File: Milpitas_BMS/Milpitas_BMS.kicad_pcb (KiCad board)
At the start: 4 copper layers, 94 x 103.4 mm, 318 parts, among them J100 JTAG, J102 DIAGS_CON, J104 CAN_CONN, J400 CHG INPUT, J401 POWER_OUTPUT, J402 BATT_PWR_INPUT, J500 SOUTH CELL CONN, J501 NORTH CELL CONN, Q400 RU1J002YNTCL, Q401 RU1J002YNTCL, Q402 RU1J002YNTCL, SW100 SW_SPST, SW101 SW_SPST, U1 BQ79606, U100 MIC5283-3.3ML-TR, U101 STM32F303RETx, U102 SN65HVD232, U200 BQ79606, U400 ACS711, U401 BTS6163DAUMA1, U402 ACS711, U403 BTS6163DAUMA1, U404 BTS6163DAUMA1, U405 ACS711, Y1 32.768kHz, Y2 32MHz

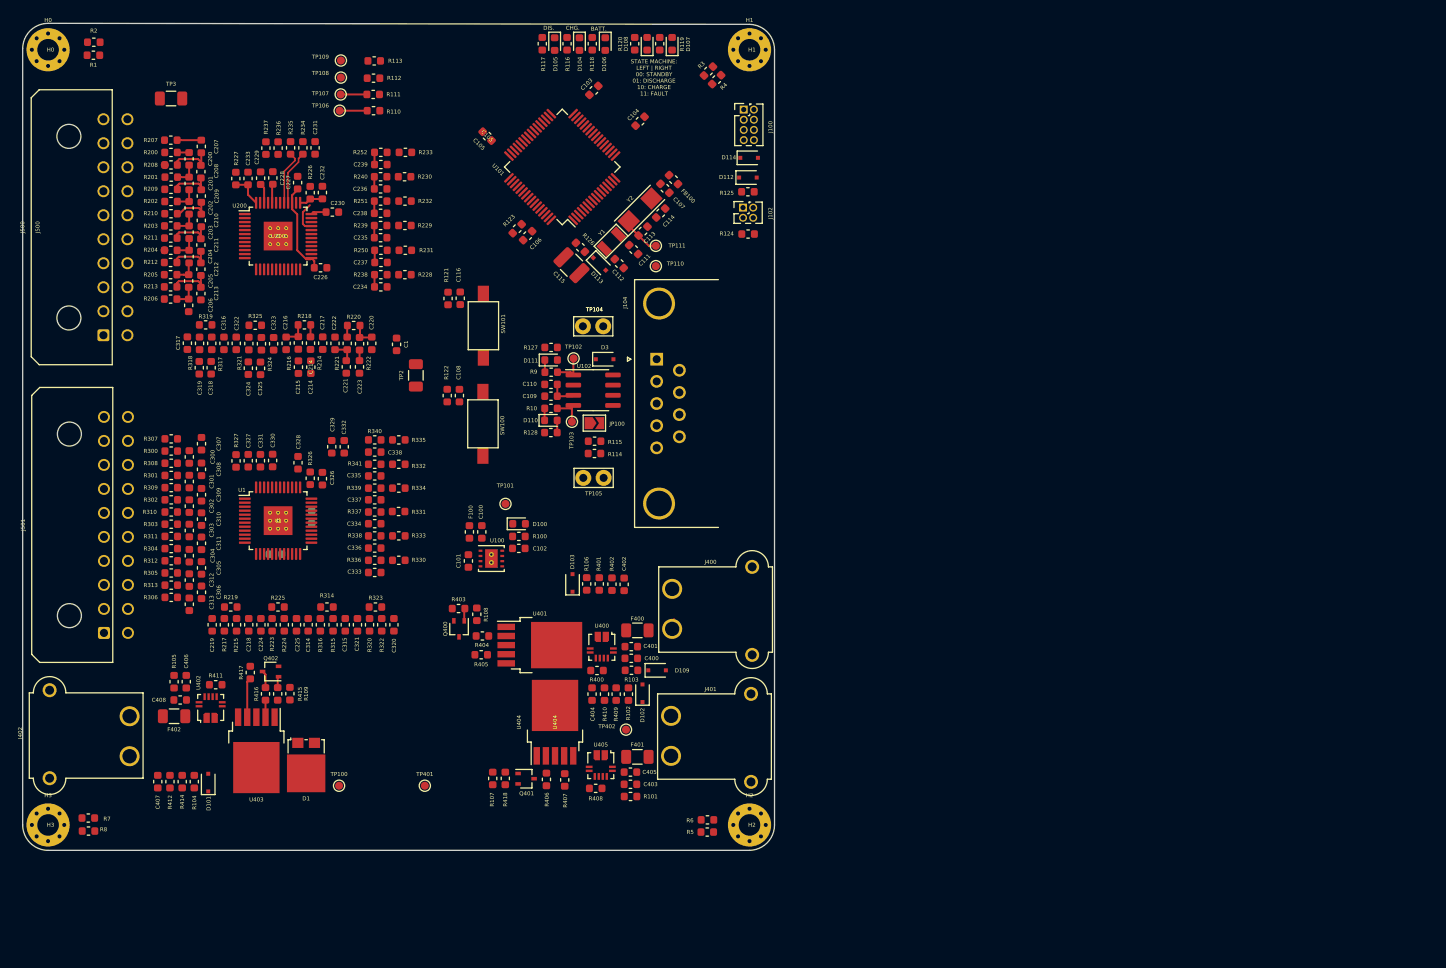
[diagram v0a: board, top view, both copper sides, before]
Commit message: First pass routing
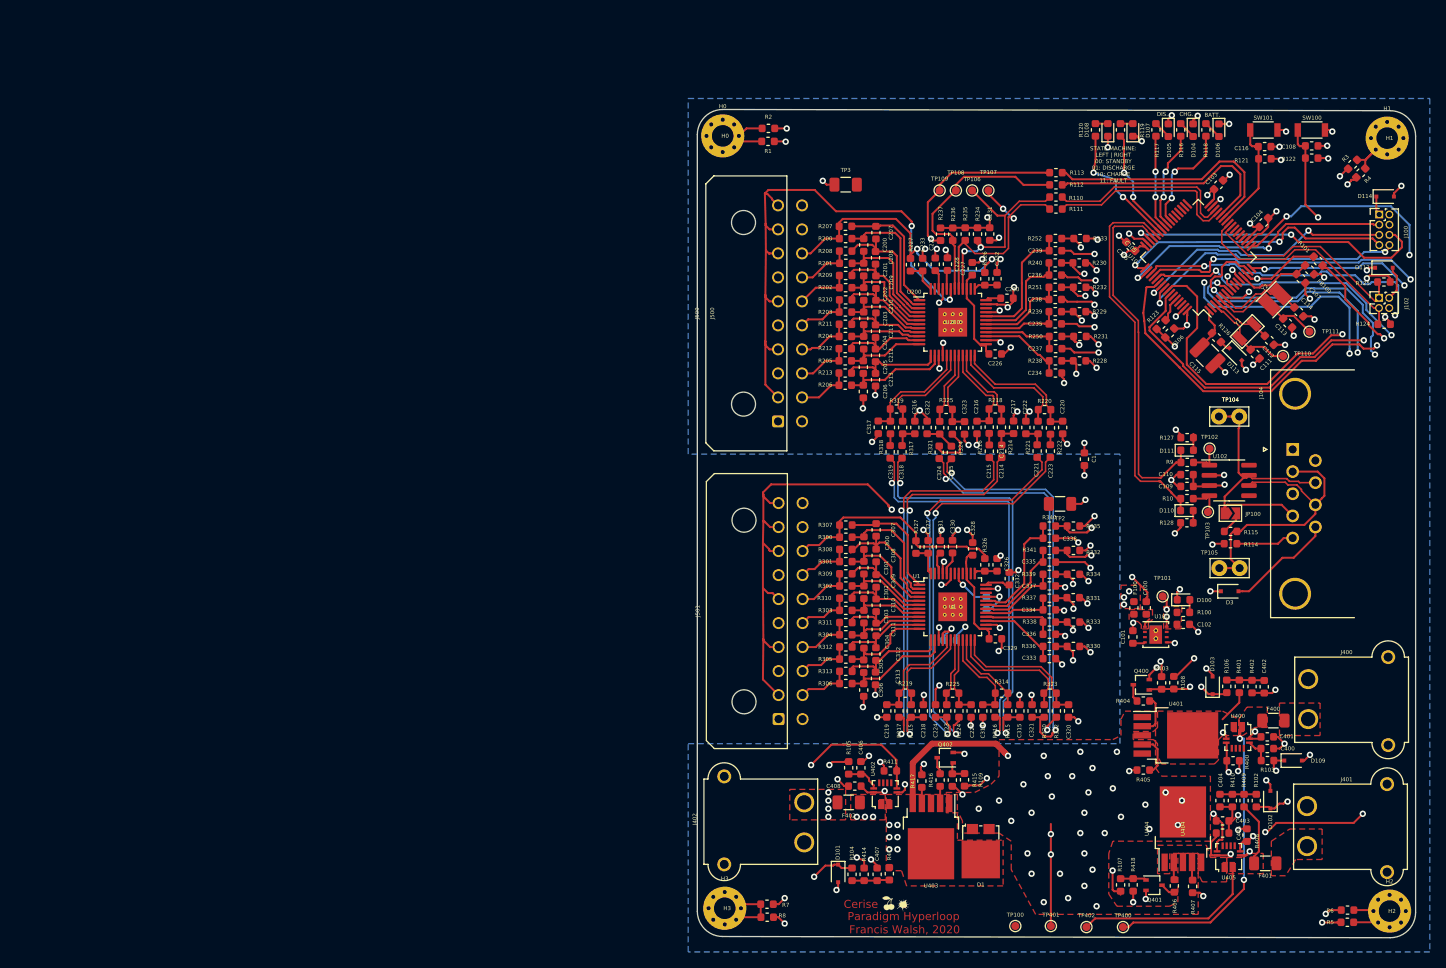
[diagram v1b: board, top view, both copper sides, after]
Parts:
- added G***: LOGO, Pics:rear_anime_ss, B.Cu at (135.4, 70.7)
- added G***: LOGO, Pics:spirograph_soldermask, F.Cu at (117.0, 146.1)
- added G***: LOGO, Pics:gunshot_logo, F.Cu at (127.3, 144.7)
- added G***: LOGO, Pics:cherry_logo, F.Cu at (125.3, 144.4)
- added TP400: CHARGER, TestPoint:TestPoint_Pad_D1.0mm, F.Cu at (154.7, 147.4)
- SW100, SW101: footprint Milpitas_BMS:KSR223GLFG -> Milpitas_BMS:B3U-1100P
- Y2: value 32MHz -> 16MHz; footprint Milpitas_BMS:NX5032GA -> Milpitas_BMS:NX3225GB
- moved R122 112.1 mm to (178.3, 51.3), turned to 180 degrees
- moved C108 111.0 mm to (178.3, 49.7), turned to 0 degrees
- moved R101 108.9 mm to (179.1, 64.1), turned to 315 degrees
- moved SW100 106.7 mm to (176.5, 47.8), turned to 0 degrees
- moved R121 103.6 mm to (172.4, 51.4), turned to 180 degrees
- moved SW101 103.5 mm to (174.0, 47.8), turned to 180 degrees
- moved C116 102.3 mm to (172.4, 49.8), turned to 0 degrees
- moved C407 90.7 mm to (124.0, 140.8), turned to 90 degrees
- moved R412 90.7 mm to (125.5, 140.7), turned to 90 degrees
- moved R403 88.4 mm to (159.5, 116.9), turned to 90 degrees
- moved R108 87.5 mm to (161.0, 116.8)
- moved C1 87.2 mm to (149.9, 88.9)
- moved C215 87.0 mm to (138.0, 87.9)
- moved C216 87.0 mm to (136.4, 84.9)
- moved C217 87.0 mm to (141.0, 84.9)
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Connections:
- C111 pad 1: /MCU/XTAL32_IN_P -> /MCU/XTAL32_P
- C112 pad 1: /MCU/XTAL32_IN_N -> /MCU/XTAL32_N
- D110 pad 1: /MCU/CAN_RX_N -> /MCU/CAN_UART_N
- D111 pad 1: /MCU/CAN_TX_P -> /MCU/CAN_UART_P
- J100 pad 2: /MCU/JTAG_TDI -> GND
- J100 pad 3: GND -> /MCU/JTAG_TDI
- J102 pad 1: /MCU/DIAGS_P -> /MCU/DIAGS_N
- J102 pad 3: /MCU/DIAGS_N -> /MCU/DIAGS_P
- J104 pad 1: Net-(D3-Pad2) -> Net-(J104-Pad1)
- J104 pad 2: /MCU/CAN_P -> /MCU/CAN_N
- J104 pad 3: /MCU/CAN_N -> Net-(J104-Pad3)
- J104 pad 6: Net-(J104-Pad6) -> GND
- J104 pad 7: Net-(J104-Pad7) -> /MCU/CAN_P
- J104 pad 9: GND -> Net-(D3-Pad2)
- J500 pad 1: Net-(J500-Pad1) -> SOUTH_THERM1_N
- J500 pad 10: Net-(J500-Pad10) -> SOUTH_THERM1_P
- J500 pad 19: Net-(J500-Pad19) -> SOUTH_THERM5_N
- J500 pad 2: Net-(J500-Pad2) -> SOUTH_THERM1_P
- J500 pad 20: Net-(J500-Pad20) -> SOUTH_THERM6_N
- J500 pad 3: Net-(J500-Pad3) -> SOUTH_THERM2_N
- J500 pad 4: Net-(J500-Pad4) -> SOUTH_THERM1_P
- J500 pad 5: Net-(J500-Pad5) -> SOUTH_THERM3_N
- J500 pad 6: Net-(J500-Pad6) -> SOUTH_THERM1_P
- J500 pad 7: Net-(J500-Pad7) -> SOUTH_THERM4_N
- J500 pad 8: Net-(J500-Pad8) -> SOUTH_THERM1_P
- J500 pad 9: Net-(J500-Pad9) -> SOUTH_THERM1_P
- J501 pad 1: NORTH_CELL_6 -> NORTH_THERM1_N
- J501 pad 11: NORTH_THERM2_N -> Net-(J501-Pad11)
- J501 pad 12: NORTH_THERM1_P -> NORTH_CELL_0
- J501 pad 13: NORTH_THERM3_N -> NORTH_CELL_1
- J501 pad 14: NORTH_THERM1_P -> NORTH_CELL_2
- J501 pad 15: NORTH_THERM4_N -> NORTH_CELL_3
- J501 pad 16: NORTH_THERM1_P -> NORTH_CELL_4
- J501 pad 17: NORTH_THERM5_N -> NORTH_CELL_5
- J501 pad 18: NORTH_THERM1_P -> NORTH_CELL_6
- J501 pad 19: NORTH_THERM6_N -> NORTH_THERM5_N
- J501 pad 2: NORTH_CELL_5 -> NORTH_THERM1_P
- J501 pad 20: Net-(J501-Pad20) -> NORTH_THERM6_N
- J501 pad 3: NORTH_CELL_5 -> NORTH_THERM2_N
- J501 pad 4: NORTH_CELL_3 -> NORTH_THERM1_P
- J501 pad 5: NORTH_CELL_2 -> NORTH_THERM3_N
- J501 pad 6: SOUTH_CELL_1 -> NORTH_THERM1_P
- J501 pad 7: NORTH_CELL_0 -> NORTH_THERM4_N
- J501 pad 9: NORTH_THERM1_N -> NORTH_THERM1_P
- R10 pad 1: /MCU/CAN_RX_N -> /MCU/CAN_UART_N
- R124 pad 1: /MCU/DIAGS_N -> /MCU/DIAGS_P
- R125 pad 1: /MCU/DIAGS_P -> /MCU/DIAGS_N
- R302 pad 2: NORTH_CELL_5 -> NORTH_CELL_4
- R305 pad 2: SOUTH_CELL_1 -> NORTH_CELL_1
- R309 pad 2: NORTH_CELL_5 -> NORTH_CELL_4
- R312 pad 2: SOUTH_CELL_1 -> NORTH_CELL_1
- R326 pad 2: +BATT -> NORTH_CELL_6
- R327 pad 2: +BATT -> NORTH_CELL_6
- R9 pad 1: /MCU/CAN_TX_P -> /MCU/CAN_UART_P
- TP110 pad 1: /MCU/XTAL32_IN_P -> /MCU/XTAL32_P
- U101 pad 14: Net-(U101-Pad14) -> /MCU/I_DIS_J
- U101 pad 15: Net-(U101-Pad15) -> /MCU/V_DIS_J
- U101 pad 16: Net-(U101-Pad16) -> /MCU/I_BATT_J
- U101 pad 17: Net-(U101-Pad17) -> /MCU/V_BATT_J
- U101 pad 24: /MCU/STM32_UART_J_N -> /MCU/DIAGS_N
- U101 pad 25: /MCU/STM32_UART_J_P -> /MCU/DIAGS_P
- U101 pad 26: Net-(U101-Pad26) -> /MCU/USR_BUTTON
- U101 pad 27: Net-(U101-Pad27) -> /MCU/BMS_WAKEUP_J
- U101 pad 28: Net-(U101-Pad28) -> /MCU/~BMS_FAULT_J
- U101 pad 29: /MCU/DIAGS_P -> /MCU/STM32_UART_J_N
- U101 pad 3: /MCU/XTAL32_IN_P -> /MCU/XTAL32_P
- U101 pad 30: /MCU/DIAGS_N -> /MCU/STM32_UART_J_P
- U101 pad 39: Net-(U101-Pad39) -> /MCU/BATT_LED
- U101 pad 4: /MCU/XTAL32_IN_N -> /MCU/XTAL32_N
- U101 pad 40: Net-(U101-Pad40) -> /MCU/CHG_LED
- U101 pad 41: Net-(U101-Pad41) -> /MCU/DIS_LED
- U101 pad 42: Net-(U101-Pad42) -> /MCU/SM0
- U101 pad 43: Net-(U101-Pad43) -> /MCU/SM1
- U101 pad 44: /MCU/CAN_RX_P -> /MCU/CAN_UART_N
- U101 pad 45: /MCU/CAN_TX_N -> /MCU/CAN_UART_P
- U101 pad 5: /MCU/XTAL32_IN_P -> /MCU/XTAL_P
- U101 pad 51: Net-(U101-Pad51) -> /MCU/BATT_ON_J
- U101 pad 52: Net-(U101-Pad52) -> BATT_FAULT
- U101 pad 53: Net-(U101-Pad53) -> /MCU/DIS_ON_J
- U101 pad 54: Net-(U101-Pad54) -> DIS_FAULT
- U101 pad 57: Net-(U101-Pad57) -> /MCU/CHG_ON_J
- U101 pad 58: Net-(U101-Pad58) -> CHG_FAULT
- U101 pad 6: /MCU/XTAL32_IN_N -> /MCU/XTAL_N
- U101 pad 8: Net-(U101-Pad8) -> /MCU/I_CHG_J
- U101 pad 9: Net-(U101-Pad9) -> /MCU/V_CHG_J
- Y1 pad 1: /MCU/XTAL32_IN_P -> /MCU/XTAL32_P
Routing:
- net BATT_FAULT: track 0.00 -> 223.7 mm, vias 0 -> 3
- net /MCU/I_BATT_J: track 0.00 -> 194.2 mm, vias 0 -> 3
- net /MCU/V_BATT_J: track 0.00 -> 186.1 mm, vias 0 -> 3
- net GND: track 0.00 -> 184.5 mm, vias 0 -> 99
- net /MCU/BATT_ON_J: track 0.00 -> 178.4 mm, vias 0 -> 3
- net /MCU/DIS_ON_J: track 0.00 -> 144.5 mm, vias 0 -> 3
- net DIS_FAULT: track 0.00 -> 120.1 mm, vias 0 -> 4
- net CHG_FAULT: track 0.00 -> 115.3 mm, vias 0 -> 2
- net /MCU/V_DIS_J: track 0.00 -> 105.0 mm, vias 0 -> 3
- net /MCU/V_CHG_J: track 0.00 -> 101.5 mm, vias 0 -> 4
- net /MCU/CHG_ON_J: track 0.00 -> 101.1 mm, vias 0 -> 2
- net I_DIS: track 0.00 -> 100.3 mm, vias 0 -> 2
- net /MCU/I_CHG_J: track 0.00 -> 96.1 mm, vias 0 -> 3
- net NORTH_THERM1_P: track 0.00 -> 70.8 mm, vias 0 -> 2
- net SOUTH_THERM1_P: track 0.00 -> 70.2 mm, vias 0 -> 2
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- added copper zone on F.Cu, net +3V3
- added copper zone on PWR, net +3V3
- added copper zone on F.Cu, net +BATT
- added copper zone on F.Cu, net /INPUT_OUTPUT/BATT_RAW
- added copper zone on F.Cu, net /INPUT_OUTPUT/CHG_MSRD
- added copper zone on F.Cu, net /INPUT_OUTPUT/CHG_RAW
- added copper zone on F.Cu, net /INPUT_OUTPUT/DIS_MSRD
- added copper zone on F.Cu, net /INPUT_OUTPUT/DIS_RAW
- added copper zone on F.Cu, net /INPUT_OUTPUT/MIXED_PWR_PLANE
- added copper zone on B.Cu, net GND
- added copper zone on GND, net GND
- added copper zone on GND, net GNDS
- added copper zone on PWR, net GNDS
- added copper zone on F.Cu, net Net-(C100-Pad1)
- added copper zone on F.Cu, net Net-(F400-Pad1)
- added copper zone on F.Cu, net Net-(F401-Pad2)
- added copper zone on F.Cu, net Net-(F402-Pad1)
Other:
- board size 94 x 103.4 mm -> 89.8 x 103.5 mm
- rule trace_min: 0.2 -> 0
- rule via_min_size: 0.4 -> 0.45
- board text added: "Cerise"
- board text added: "Francis Walsh, 2020"
- board text added: "Paradigm Hyperloop"
